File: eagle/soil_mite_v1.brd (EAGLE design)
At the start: 100 x 80 mm, 30 parts, among them U4 TEMP_SENSOR_LMT84, U5 TRISTATE_BUFFER_SOT353, X1 1365-10

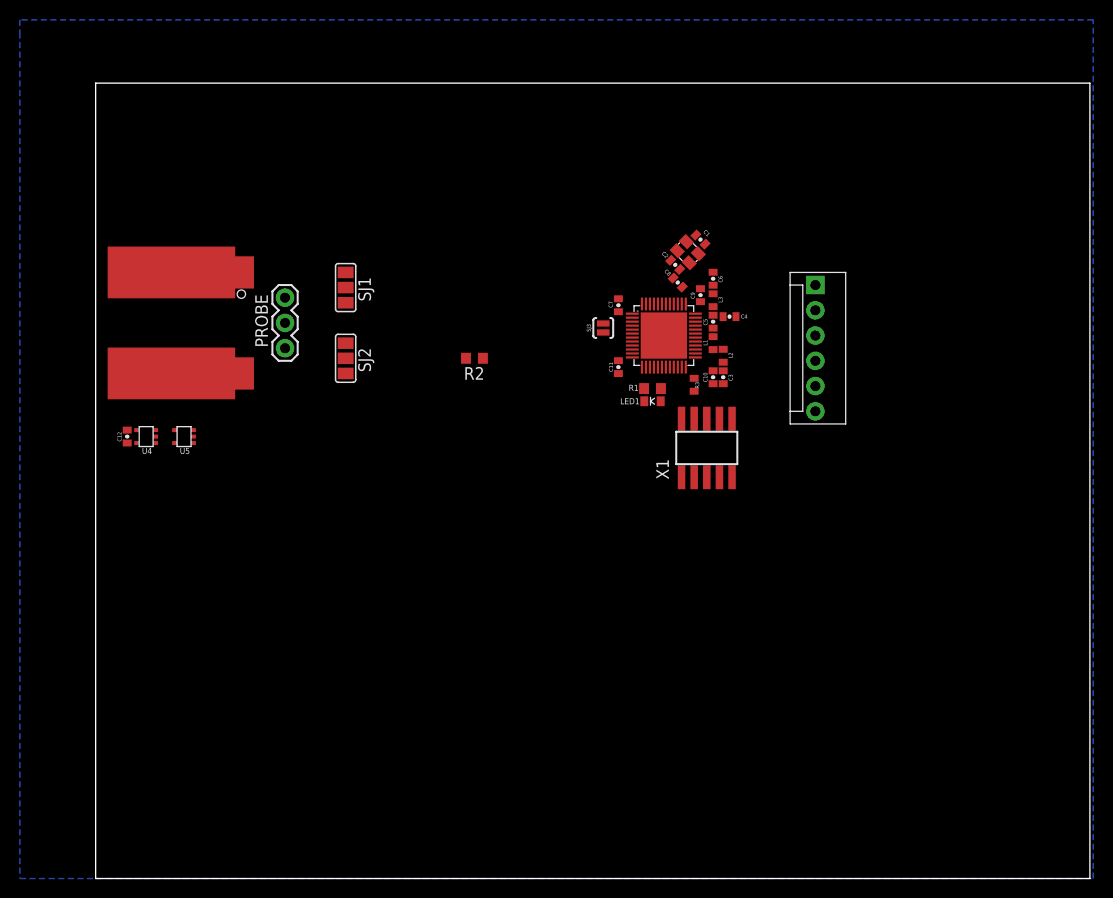
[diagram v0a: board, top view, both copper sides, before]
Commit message: finished layout. let me know if there are glaring errors
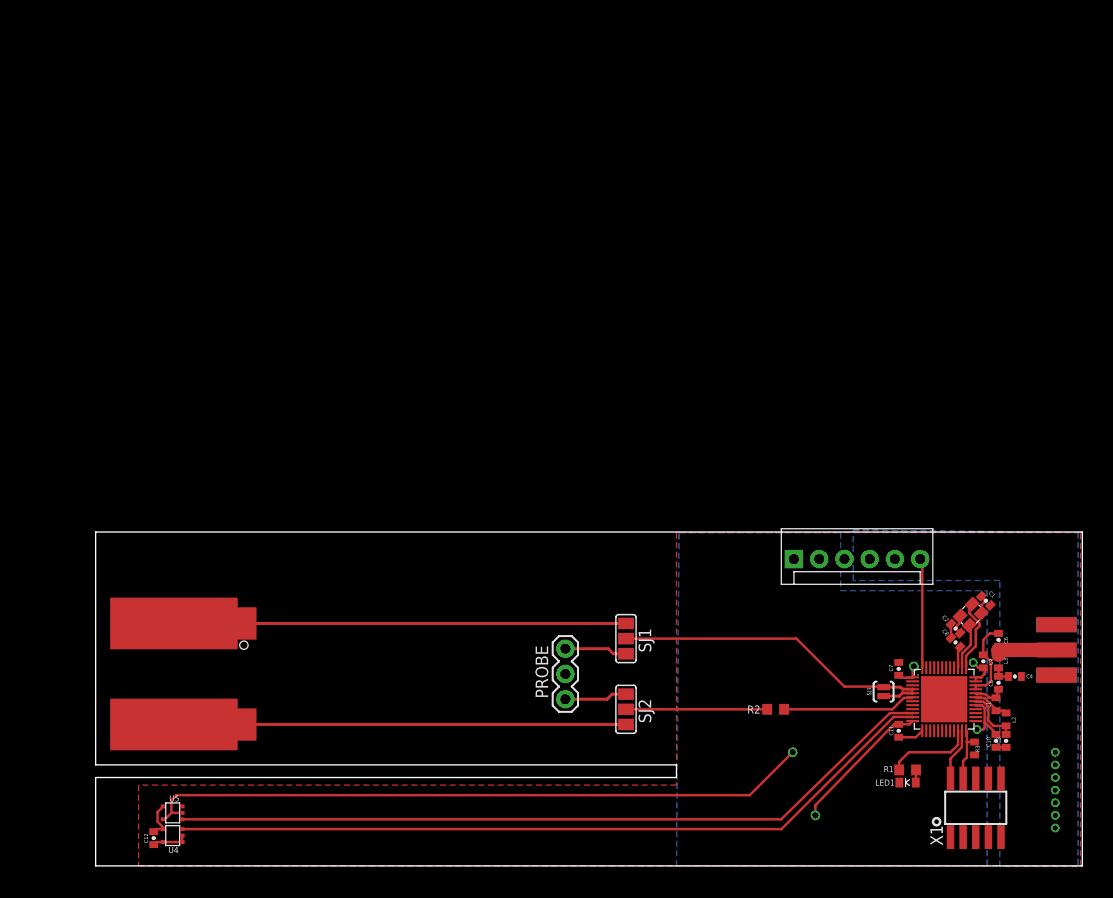
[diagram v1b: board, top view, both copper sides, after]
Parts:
- added J$1: SMA_EDGE, SparkFun-Connectors:SMA-EDGE
- moved C9 46.5 mm to (89.3, 21.8)
- moved R2 46.5 mm to (68.4, 17.0)
- moved L2 46.3 mm to (91.6, 16.0), turned to 270 degrees
- moved C10 46.3 mm to (90.6, 13.8), turned to 270 degrees
- moved C3 46.3 mm to (91.6, 13.8), turned to 270 degrees
- moved C5 46.3 mm to (90.8, 19.7)
- moved C6 46.3 mm to (90.8, 24.0)
- moved C1 46.3 mm to (89.5, 27.9)
- moved L3 46.3 mm to (90.8, 21.8)
- moved U$2 46.2 mm to (88.0, 26.5), turned to 45 degrees
- moved C4 46.2 mm to (92.5, 20.3)
- moved C11 46.2 mm to (80.8, 14.9)
- moved C7 46.2 mm to (80.8, 21.1)
- moved SJ3 46.2 mm to (79.2, 18.8)
- moved C2 46.2 mm to (86.5, 25.1)
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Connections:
- net ANTENNA: now also J$1.SIG
- net GND: now also J$1.GND@0, J$1.GND@1, J$1.GND@2, J$1.GND@3
- net XC1: now also U$2.X2; no longer U$2.X1
- net XC2: now also U$2.X1; no longer U$2.X2
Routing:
- net +1V8: track 0.00 -> 93.9 mm, vias 0 -> 5
- net TEMP: track 0.00 -> 78.2 mm
- net TEMP_EN: track 0.00 -> 77.8 mm
- net SOIL_PWM_JUNC1: track 0.00 -> 40.4 mm
- net FROMSOIL_CAP_JUNC1: track 0.00 -> 40.4 mm
- net SOIL_PWM: track 0.00 -> 30.9 mm
- net FROMSOIL_CAP: track 0.00 -> 27.6 mm
- net GND: track 0.00 -> 17.1 mm, vias 0 -> 7
- net VREADY: track 0.00 -> 11.0 mm
- net INDICATOR: track 0.00 -> 8.85 mm
- net XC1: track 0.00 -> 7.49 mm
- net SWDCLK: track 0.00 -> 7.10 mm
- net ANTENNA: track 0.00 -> 6.70 mm
- net FROMSOIL_CAP_JUNC2: track 0.00 -> 6.31 mm
- net SOIL_PWM_JUNC2: track 0.00 -> 6.31 mm
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- added copper zone on layer 16, net +1V8
- added copper zone on layer 1, net GND
- added copper zone on layer 16, net GND
- removed copper zone on layer 16, net N$1
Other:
- board size 100 x 80 mm -> 99.2 x 33.6 mm
